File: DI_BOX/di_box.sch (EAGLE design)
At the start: 10 parts, among them Q1 2N5950, X1 MC3FAH-0

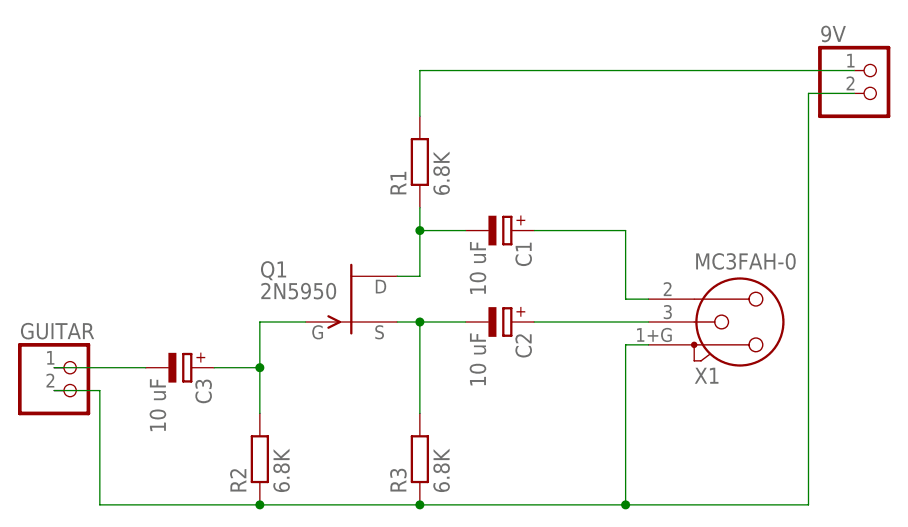
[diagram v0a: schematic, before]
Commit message: updated schematic
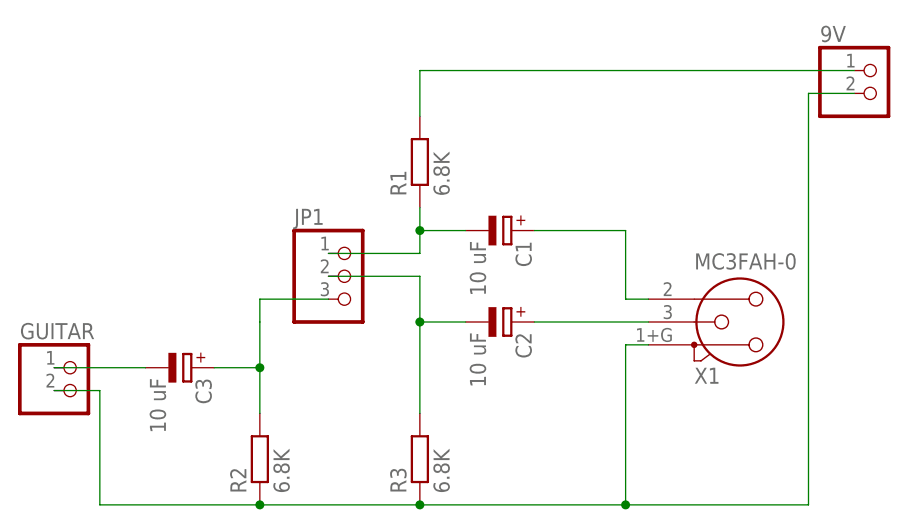
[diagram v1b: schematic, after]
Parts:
- removed Q1: 2N5950, transistor-fet:2N5950
- added JP1: (no value), pinhead:PINHD-1X3
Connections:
- net N$1: now also JP1.3; no longer Q1.G
- net N$2: now also JP1.1; no longer Q1.D
- net N$4: now also JP1.2; no longer Q1.S
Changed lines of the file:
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@@
 <part name="C2" library="rcl" library_urn="urn:adsk.eagle:library:334" deviceset="CPOL-EU" device="E2-4" package3d_urn="urn:adsk.eagle:package:23347/1" value="10 uF"/>
 <part name="C3" library="rcl" library_urn="urn:adsk.eagle:library:334" deviceset="CPOL-EU" device="E2-4" package3d_urn="urn:adsk.eagle:package:23347/1" value="10 uF"/>
-<part name="Q1" library="transistor-fet" library_urn="urn:adsk.eagle:library:396" deviceset="2N5950" device="" package3d_urn="urn:adsk.eagle:package:28535/2"/>
 <part name="9V" library="pinhead" library_urn="urn:adsk.eagle:library:325" deviceset="PINHD-1X2" device="" package3d_urn="urn:adsk.eagle:package:22435/2"/>
 <part name="X1" library="con-neutrik_ag" library_urn="urn:adsk.eagle:library:166" deviceset="MC3?" device="FAH-0" package3d_urn="urn:adsk.eagle:package:8886/1"/>
 <part name="GUITAR" library="pinhead" library_urn="urn:adsk.eagle:library:325" deviceset="PINHD-1X2" device="" package3d_urn="urn:adsk.eagle:package:22435/2"/>
+<part name="JP1" library="pinhead" library_urn="urn:adsk.eagle:library:325" deviceset="PINHD-1X3" device="" package3d_urn="urn:adsk.eagle:package:22458/2"/>
 </parts>
 <sheets>
@@
 <instance part="C2" gate="G$1" x="53.34" y="53.34" rot="R270"/>
 <instance part="C3" gate="G$1" x="17.78" y="48.26" rot="R270"/>
-<instance part="Q1" gate="G$1" x="35.56" y="55.88"/>
 <instance part="9V" gate="G$1" x="93.98" y="78.74"/>
 <instance part="X1" gate="G$1" x="78.74" y="53.34" rot="MR180"/>
 <instance part="GUITAR" gate="G$1" x="5.08" y="45.72"/>
+<instance part="JP1" gate="A" x="35.56" y="58.42"/>
 </instances>
 <busses>
@@
 <pinref part="R2" gate="G$1" pin="2"/>
 <wire x1="25.4" y1="48.26" x2="25.4" y2="43.18" width="0.1524" layer="91"/>
-<pinref part="Q1" gate="G$1" pin="G"/>
 <wire x1="25.4" y1="48.26" x2="25.4" y2="53.34" width="0.1524" layer="91"/>
-<wire x1="25.4" y1="53.34" x2="30.48" y2="53.34" width="0.1524" layer="91"/>
 <junction x="25.4" y="48.26"/>
+<pinref part="JP1" gate="A" pin="3"/>
+<wire x1="25.4" y1="53.34" x2="25.4" y2="55.88" width="0.1524" layer="91"/>
+<wire x1="25.4" y1="55.88" x2="33.02" y2="55.88" width="0.1524" layer="91"/>
 </segment>
 </net>
@@
 <net name="N$4" class="0">
 <segment>
-<pinref part="Q1" gate="G$1" pin="S"/>
 <pinref part="R3" gate="G$1" pin="2"/>
-<wire x1="40.64" y1="53.34" x2="43.18" y2="53.34" width="0.1524" layer="91"/>
 <wire x1="43.18" y1="53.34" x2="43.18" y2="43.18" width="0.1524" layer="91"/>
 <pinref part="C2" gate="G$1" pin="-"/>
 <wire x1="43.18" y1="53.34" x2="48.26" y2="53.34" width="0.1524" layer="91"/>
+<wire x1="43.18" y1="53.34" x2="43.18" y2="58.42" width="0.1524" layer="91"/>
 <junction x="43.18" y="53.34"/>
+<pinref part="JP1" gate="A" pin="2"/>
+<wire x1="43.18" y1="58.42" x2="33.02" y2="58.42" width="0.1524" layer="91"/>
 </segment>
 </net>
 <net name="N$2" class="0">
 <segment>
-<pinref part="Q1" gate="G$1" pin="D"/>
-<wire x1="40.64" y1="58.42" x2="43.18" y2="58.42" width="0.1524" layer="91"/>
 <pinref part="R1" gate="G$1" pin="1"/>
-<wire x1="43.18" y1="58.42" x2="43.18" y2="63.5" width="0.1524" layer="91"/>
 <pinref part="C1" gate="G$1" pin="-"/>
 <wire x1="43.18" y1="63.5" x2="43.18" y2="66.04" width="0.1524" layer="91"/>
 <wire x1="48.26" y1="63.5" x2="43.18" y2="63.5" width="0.1524" layer="91"/>
+<pinref part="JP1" gate="A" pin="1"/>
+<wire x1="43.18" y1="63.5" x2="43.18" y2="60.96" width="0.1524" layer="91"/>
+<wire x1="43.18" y1="60.96" x2="33.02" y2="60.96" width="0.1524" layer="91"/>
 <junction x="43.18" y="63.5"/>
 </segment>
